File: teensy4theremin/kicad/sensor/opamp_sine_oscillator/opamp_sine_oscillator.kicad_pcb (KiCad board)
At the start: 2 copper layers, 28 parts, among them J1 L_IN, J2 L_OUT, J3 ANTENNA, J4 Conn_01x03_Male, U1 AD8052ARZ, U2 MCP1700-3302E_SOT23, U3 SP721

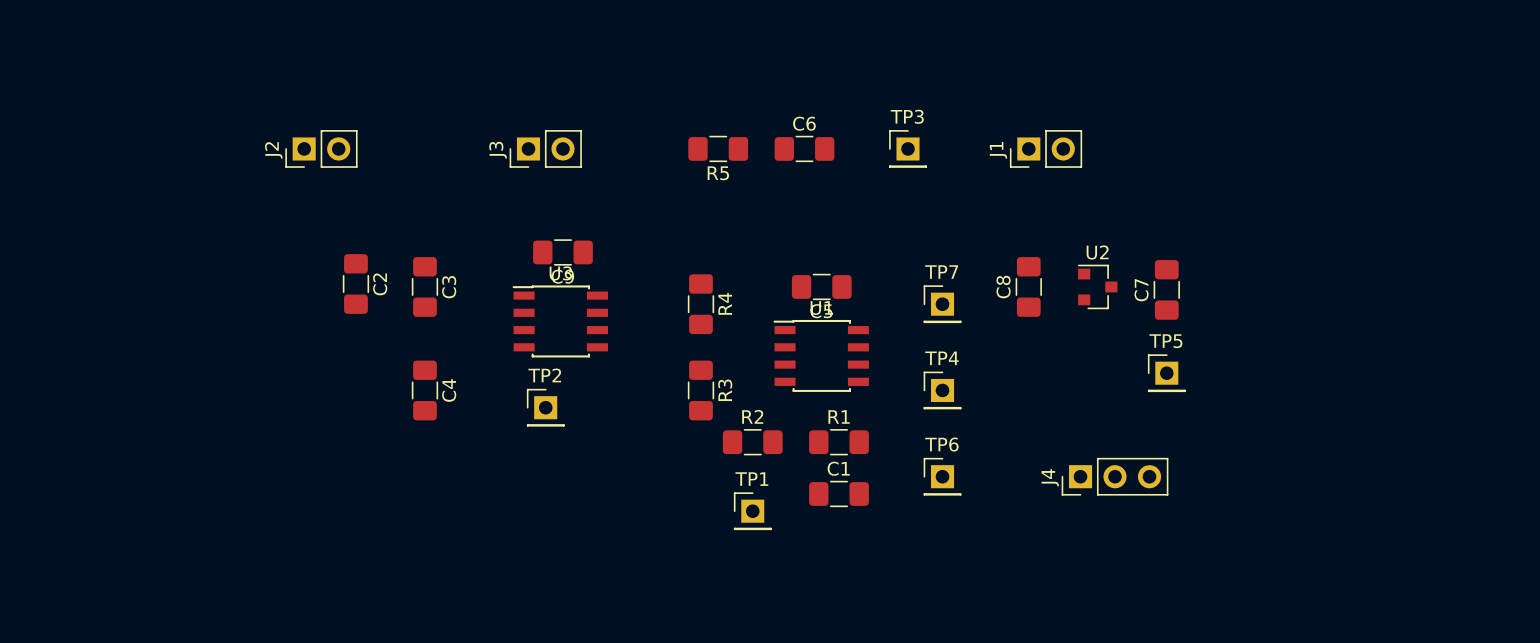
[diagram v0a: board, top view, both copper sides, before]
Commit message: oscillator PCB
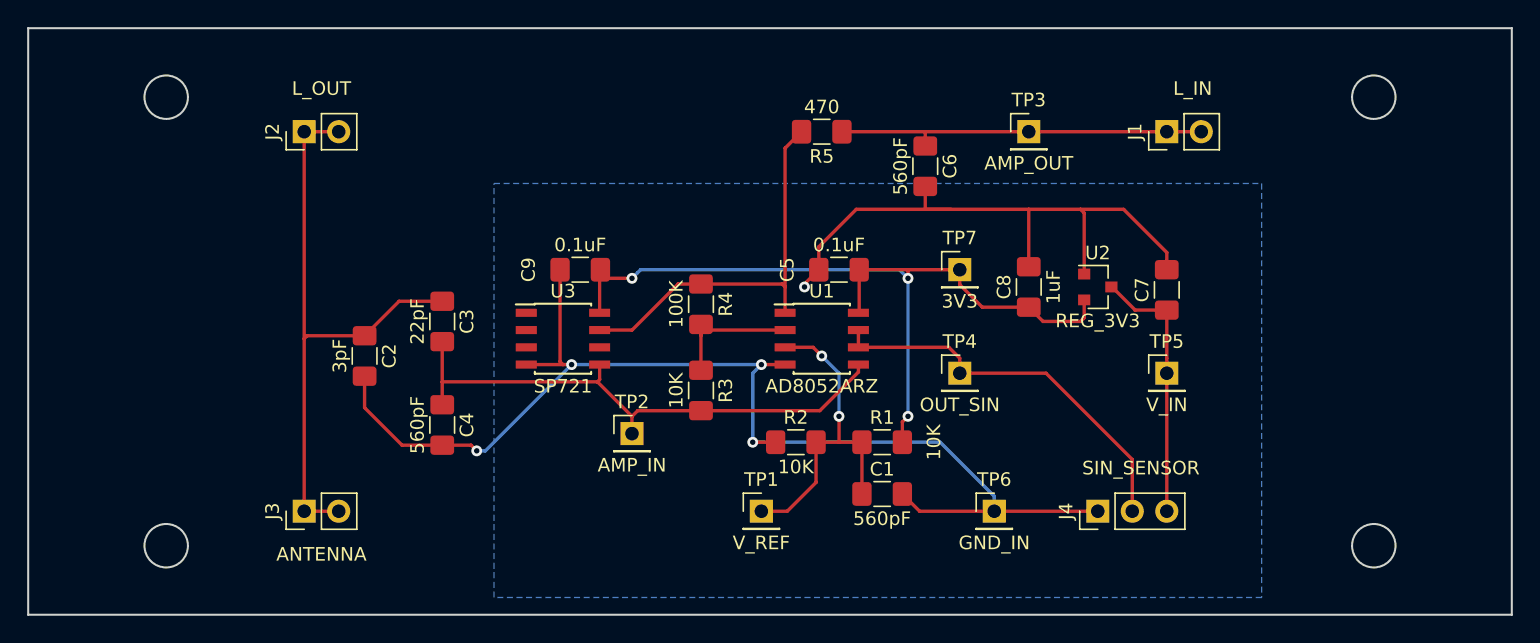
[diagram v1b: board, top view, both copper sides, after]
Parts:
- J4: value Conn_01x03_Male -> SIN_SENSOR
- TP1: value TestPoint -> V_REF
- TP2: value TestPoint -> AMP_IN
- TP3: value TestPoint -> AMP_OUT
- TP4: value TestPoint -> OUT_SIN
- TP5: value TestPoint -> V_IN
- TP6: value TestPoint -> GND_IN
- TP7: value TestPoint -> 3V3
- U2: value MCP1700-3302E_SOT23 -> REG_3V3
- moved J3 31.4 mm to (63.5, 114.3)
- moved J1 10.2 mm to (127.0, 86.4)
- moved C6 8.98 mm to (109.2, 88.9), turned to 270 degrees
- moved TP3 8.98 mm to (116.8, 86.4)
- moved R5 7.73 mm to (101.6, 86.4)
- moved TP2 6.63 mm to (87.6, 108.6)
- moved C2 5.34 mm to (67.9, 102.9)
- moved TP6 4.58 mm to (114.3, 114.3)
- moved C1 3.17 mm to (106.0, 113.0)
- moved R1 3.17 mm to (106.0, 109.2)
- moved R2 3.17 mm to (99.7, 109.2)
- moved TP7 2.84 mm to (111.8, 96.5)
- moved C4 2.84 mm to (73.7, 108.0)
- moved C3 2.84 mm to (73.7, 100.3)
- moved J4 2.84 mm to (121.9, 114.3)
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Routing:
- net GND: track 0.00 -> 136.2 mm, vias 0 -> 5
- net +3V3: track 0.00 -> 62.9 mm, vias 0 -> 3
- net Net-(C2-Pad1): track 0.00 -> 44.3 mm
- net /ESD1: track 0.00 -> 40.8 mm
- net Net-(J4-Pad2): track 0.00 -> 29.3 mm
- net /ESD2: track 0.00 -> 29.0 mm
- net Net-(C6-Pad1): track 0.00 -> 27.5 mm
- net /VREF: track 0.00 -> 24.9 mm, vias 0 -> 2
- net +5V: track 0.00 -> 19.6 mm
- net Net-(R3-Pad1): track 0.00 -> 8.93 mm
- added copper zone on B.Cu, net GND
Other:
- board outline added: 109.2 x 43.2 mm
